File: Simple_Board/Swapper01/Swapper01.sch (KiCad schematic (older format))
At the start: 35 parts, among them J1 DB9_Female_MountingHoles

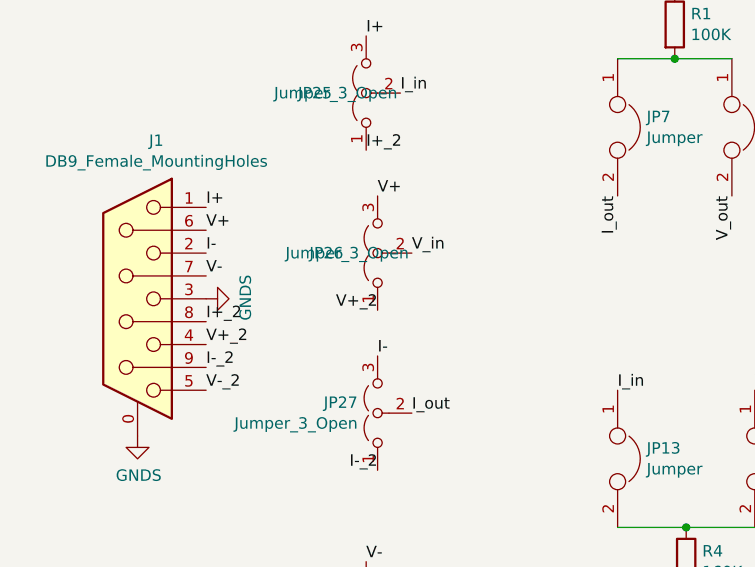
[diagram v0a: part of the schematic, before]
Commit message: Upddate
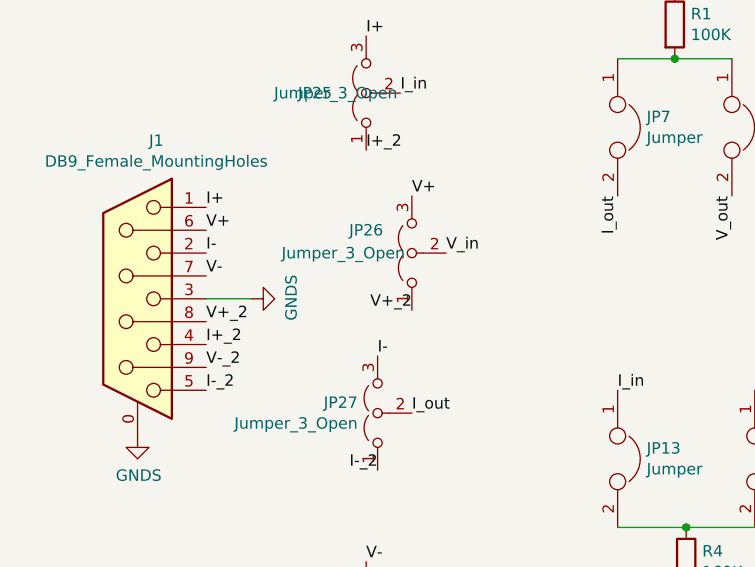
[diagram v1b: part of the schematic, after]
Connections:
- net I+_2: now also J1.4; no longer J1.8
- net I-_2: now also J1.5; no longer J1.9
- net V+_2: now also J1.8; no longer J1.4
- net V-_2: now also J1.9; no longer J1.5
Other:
- moved on the sheet: JP26
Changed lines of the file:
@@
 Text Label 1100 2600 0    50   ~ 0
 V-
+Text Label 1100 2900 0    50   ~ 0
+I+_2
 Text Label 1100 2800 0    50   ~ 0
-I+_2
-Text Label 1100 2900 0    50   ~ 0
 V+_2
+Text Label 1100 3100 0    50   ~ 0
+I-_2
 Text Label 1100 3000 0    50   ~ 0
-I-_2
-Text Label 1100 3100 0    50   ~ 0
 V-_2
 $Comp
@@
 Text Label 1800 2050 0    50   ~ 0
 I+_2
-Text Label 1850 2250 0    50   ~ 0
+Text Label 2000 2250 0    50   ~ 0
 V+
-Text Label 1850 2750 2    50   ~ 0
+Text Label 2000 2750 2    50   ~ 0
 V+_2
 Text Label 1850 2950 0    50   ~ 0
@@
 L Jumper:Jumper_3_Open JP26
 U 1 1 6280857B
-P 1850 2500
-F 0 "JP26" V 1850 2724 50  0000 C CNN
-F 1 "Jumper_3_Open" V 1850 2633 50  0000 C CNN
-F 2 "Jumper:SolderJumper-3_P1.3mm_Open_Pad1.0x1.5mm" H 1850 2500 50  0001 C CNN
-F 3 "~" H 1850 2500 50  0001 C CNN
-	1    1850 2500
+P 2000 2500
+F 0 "JP26" V 2100 2700 50  0000 C CNN
+F 1 "Jumper_3_Open" V 2000 2800 50  0000 C CNN
+F 2 "Jumper:SolderJumper-3_P1.3mm_Open_Pad1.0x1.5mm" H 2000 2500 50  0001 C CNN
+F 3 "~" H 2000 2500 50  0001 C CNN
+	1    2000 2500
 	0    -1   -1   0
 $EndComp
@@
 Text Label 1950 1800 0    50   ~ 0
 I_in
-Text Label 2000 2500 0    50   ~ 0
+Text Label 2150 2500 0    50   ~ 0
 V_in
 Text Label 2000 3200 0    50   ~ 0
@@
 I_out
 $Comp
-L power:GNDS #PWR?
+L power:GNDS #PWR0101
 U 1 1 62838416
-P 1100 2700
-F 0 "#PWR?" H 1100 2450 50  0001 C CNN
-F 1 "GNDS" H 1105 2527 50  0000 C CNN
-F 2 "" H 1100 2700 50  0001 C CNN
-F 3 "" H 1100 2700 50  0001 C CNN
-	1    1100 2700
-	0    -1   -1   0
-$EndComp
+P 1300 2700
+F 0 "#PWR0101" H 1300 2450 50  0001 C CNN
+F 1 "GNDS" H 1305 2527 50  0000 C CNN
+F 2 "" H 1300 2700 50  0001 C CNN
+F 3 "" H 1300 2700 50  0001 C CNN
+	1    1300 2700
+	0    -1   -1   0
+$EndComp
+Wire Wire Line
+	1100 2700 1300 2700
 $EndSCHEMATC

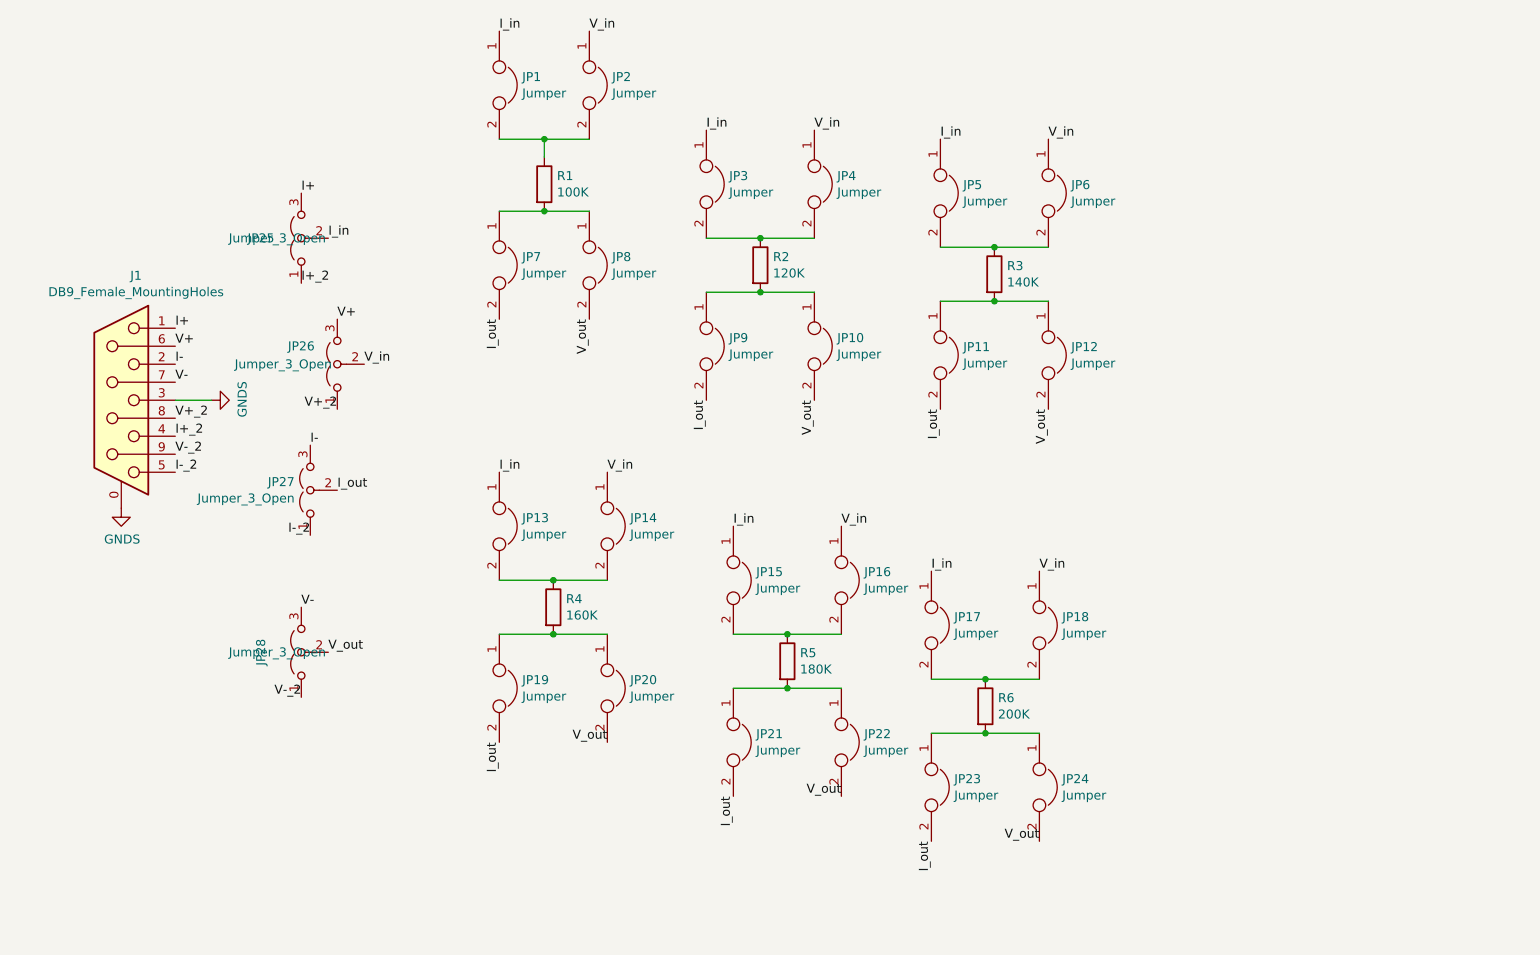
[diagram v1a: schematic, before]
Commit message: Update
Nearly finished versions of simple and Calibrator board
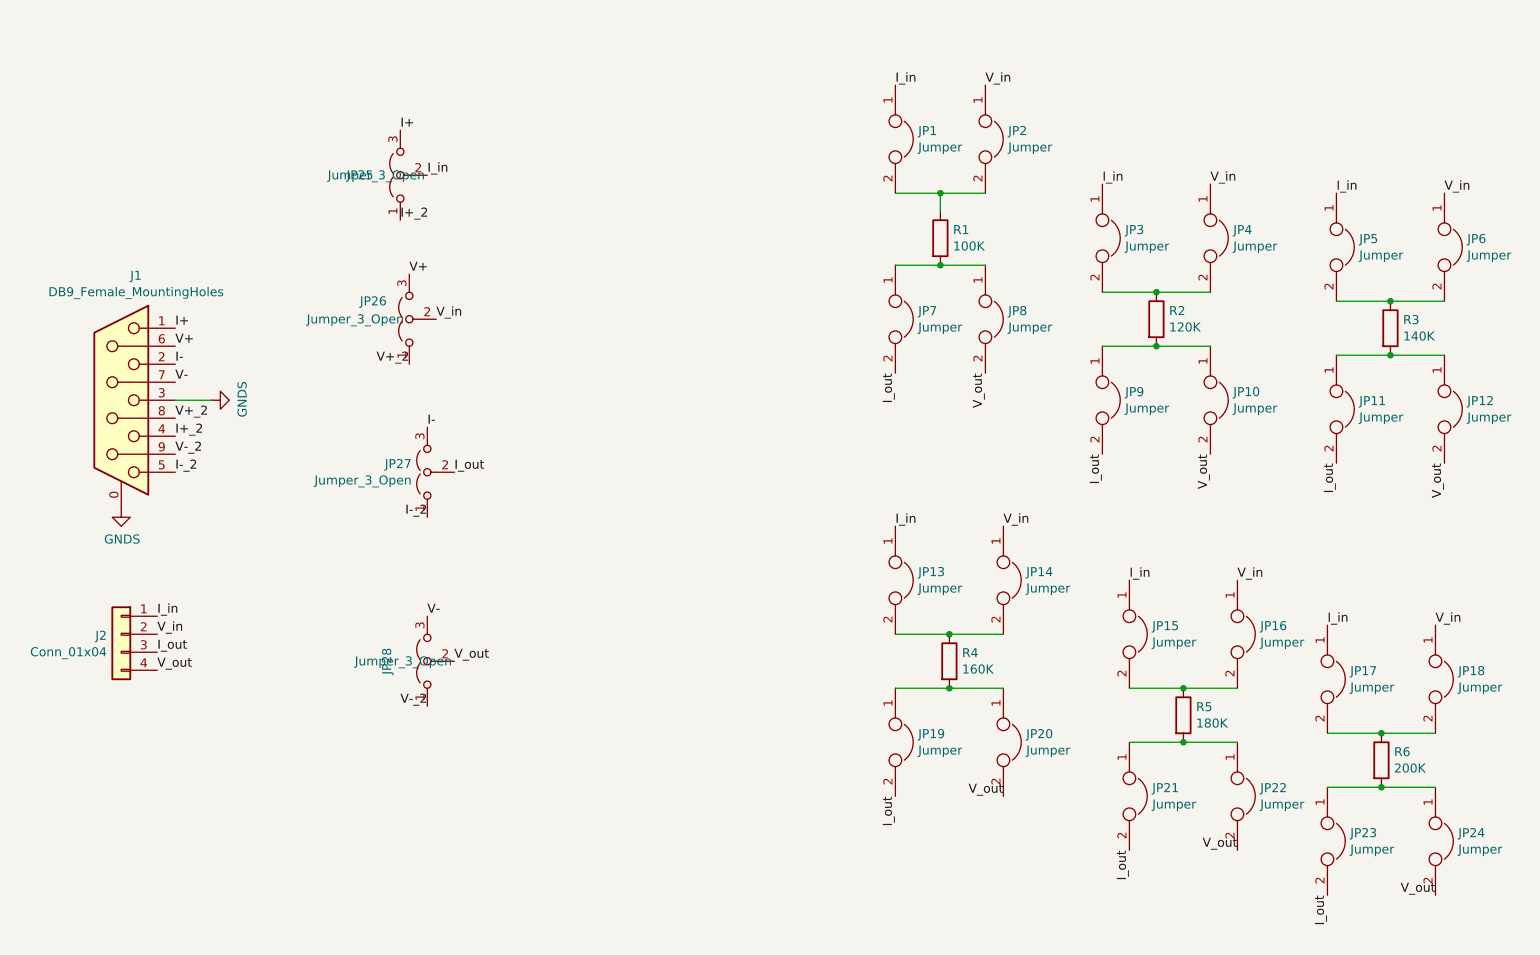
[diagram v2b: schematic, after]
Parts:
- added J2: Conn_01x04, Connector_JST:JST_SH_SM04B-SRSS-TB_1x04-1MP_P1.00mm_Horizontal, symbol Connector_Generic:Conn_01x04
- J1: footprint Connector:DB9_ASSMANN -> 0_Swapper01:DSUB-TH_DMR-9S; LCSC (none) -> C141882
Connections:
- net I_in: now also J2.1 (Pin_1)
- net I_out: now also J2.3 (Pin_3)
- net V_in: now also J2.2 (Pin_2)
- net V_out: now also J2.4 (Pin_4)
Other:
- moved on the sheet: JP1, JP10, JP11, JP12, JP13, JP14, JP15, JP16, JP17, JP18, JP19, JP2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
